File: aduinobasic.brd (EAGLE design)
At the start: 96 parts

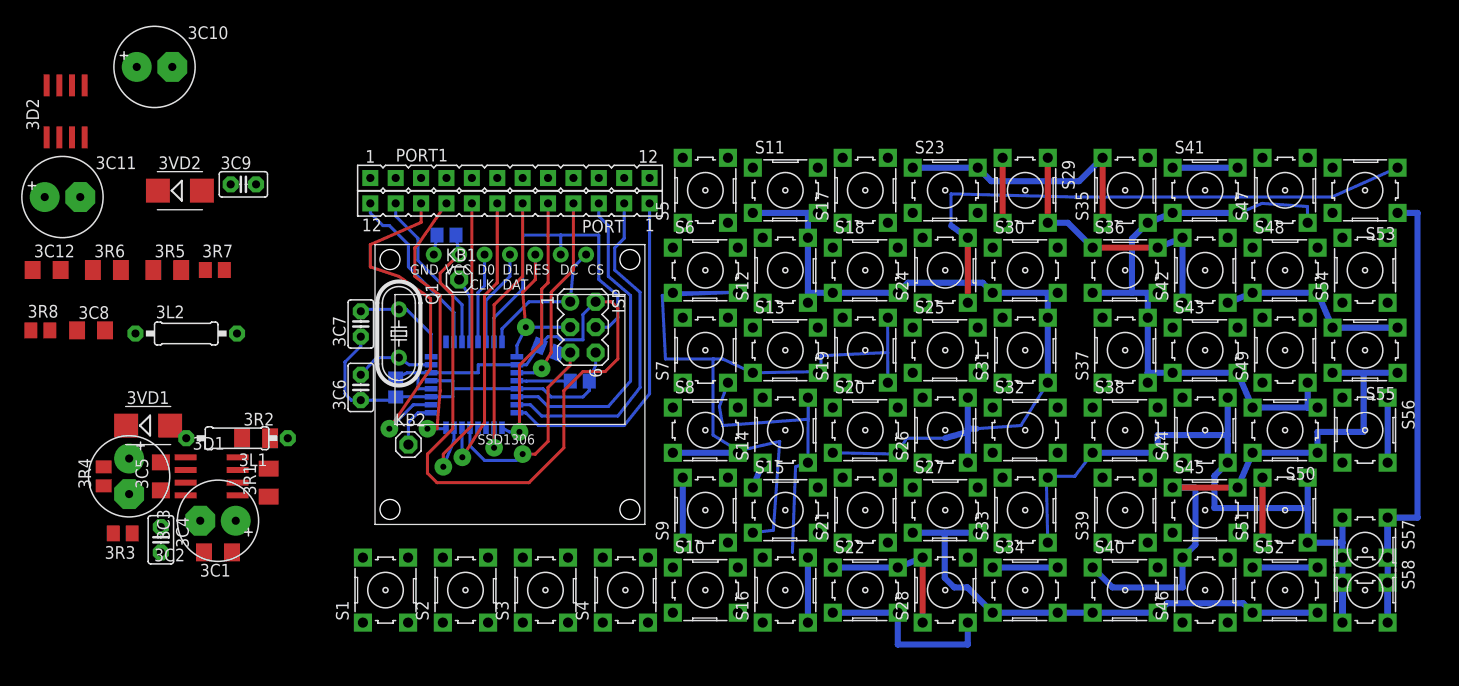
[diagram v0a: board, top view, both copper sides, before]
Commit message: .
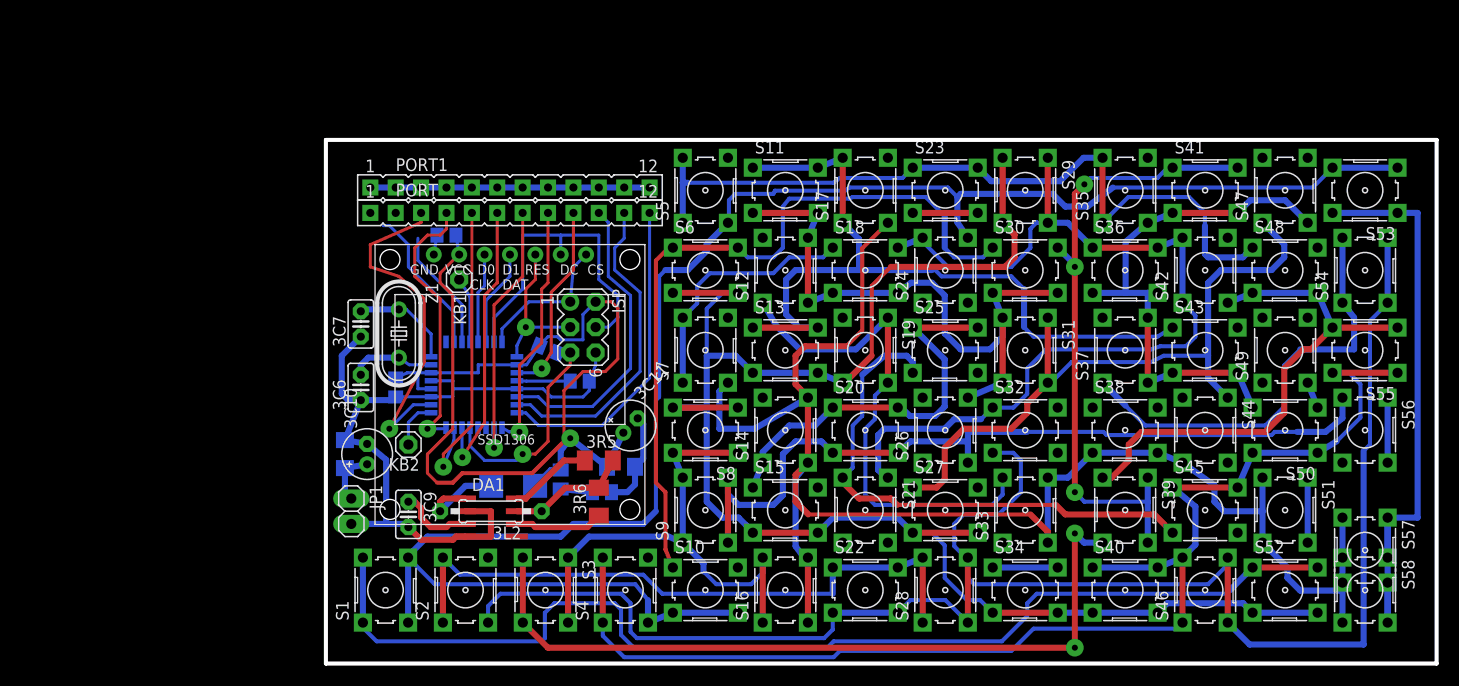
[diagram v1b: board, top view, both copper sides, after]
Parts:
- removed 3C1: 100n, rc-elektronik:C1206
- removed 3C2: 470µ / 10V, HWProgUSB:RCL_E3,5-8
- removed 3C3: 100µ 16V, HWProgUSB:RCL_E3,5-8
- removed 3C4: 1n, rcl:C025-025X050
- removed 3C5: 100n, rcl:C1206
- removed 3D1, 3D2: MC34063AD, mc34063:SOIC8
- removed 3L1: 100uh, rcl:0207/10
- removed 3R1: 0.5-1, rcl:M1206
- removed 3R2: 220, rcl:M1206
- removed 3R3: 2k2, rcl:M0805
- removed 3R4: 20k, rcl:M0805
- removed 3VD1: SS12, diode:SMB
- added DA1: MC34063AD, mc34063:SOIC8
- added JP1: (no value), pinhead:1X02
- 3C10, 3C11: device HWProgUSB:RCL_E3,5-8 -> HWProgUSB:RCL_E2-5
- 3R5: value 220 -> 180
- 3R6: value 0.5-1 -> 1
- 3R7: value 20k -> 3k
- 3R8: value 2k2 -> 1k
- C1, C2, C3: value (none) -> 100n
- Z1: value (none) -> 16Mhz
- moved 3C11 61.3 mm to (56.5, 37.5), turned to 45 degrees
- moved 3C12 60.7 mm to (55.6, 33.3), flipped to the bottom
- moved 3R8 58.5 mm to (53.7, 30.8), flipped to the bottom
- moved 3R6 54.4 mm to (53.3, 29.8), turned to 90 degrees
- moved 3R5 47.2 mm to (53.3, 34.0)
- moved 3VD2 44.5 mm to (44.8, 31.4), flipped to the bottom
- moved 3C10 44.2 mm to (30.2, 34.6), turned to 90 degrees
- moved 3R7 40.5 mm to (49.5, 32.1), flipped to the bottom, turned to 90 degrees
- moved 3C9 36.9 mm to (34.3, 28.6), turned to 270 degrees
- moved 3L2 35.3 mm to (42.5, 28.9), turned to 180 degrees
- moved 3C8 28.3 mm to (27.9, 34.6), flipped to the bottom, turned to 90 degrees
- moved PORT 0.95 mm to (44.5, 58.7), turned to 0 degrees
- moved PORT1 0.95 mm to (44.5, 61.3)
- turned S19 to 270 degrees
- turned S21 to 270 degrees
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- renumbered Q1 to Z1
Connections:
- removed net +12V: 3C11.+, 3C12.2, 3C3.+, 3C5.2, 3R4.2, 3R7.2, 3VD1.C, 3VD2.C
- removed net +5V: 3C1.1, 3C10.+, 3C2.+, 3C8.1, 3D1.6, 3D2.6, 3R1.1, 3R6.1
- removed net N$104: 3D1.8, 3R2.1
- removed net N$105: 3D1.7, 3L1.1, 3R1.2, 3R2.2
- removed net N$106: 3D1.5, 3R3.2, 3R4.1
- removed net N$107: 3D1.1, 3L1.2, 3VD1.A
- removed net N$108: 3C4.1, 3D1.3
- new net V+: 3C10.+, 3C8.1, 3R6.1, DA1.6, JP1.1
- net A0: now also PORT.11; no longer PORT.2
- net A1: now also PORT.12; no longer PORT.1
- net A2: now also PORT.8; no longer PORT.5
- net A3: now also PORT.7; no longer PORT.6
- net A6: now also PORT.9; no longer PORT.4
- net A7: now also PORT.10; no longer PORT.3
- net D0: now also PORT.6; no longer PORT.7
- net D1: now also PORT.5; no longer PORT.8
- net D12: now also S16.2, S3.2, S54.2, S8.2
- net D13: now also S11.2, S13.2, S17.2
- net D14: now also S19.2, S33.2
- net D15: now also S18.2, S21.2, S24.2, S7.2; no longer S24.1
- net D16: now also S20.2, S25.2, S5.2
- net D17: now also S30.2, S39.2, S6.2
- net D18: now also S31.2
- net D19: now also S4.2, S40.2
- net D2: now also PORT.4; no longer PORT.9
- net D23: now also S2.2
- net D26: now also S1.2
- net D3: now also S53.2
- net D4: now also PORT.3; no longer PORT.10
- net D6: now also PORT.1; no longer PORT.12
- net D7: now also PORT.2; no longer PORT.11
- net GND: now also DA1.2, DA1.4, JP1.2, PORT1.1, PORT1.10, PORT1.11, PORT1.12, PORT1.2, PORT1.3, PORT1.4, PORT1.5, PORT1.6, PORT1.7, PORT1.8, PORT1.9; no longer 3C1.2, 3C2.-, 3C3.-, 3C4.2, 3C5.1, 3D1.2, 3D1.4, 3D2.2, 3D2.4, 3R3.1
- net N$5: now also DA1.8; no longer 3D2.8
- net N$6: now also DA1.7; no longer 3D2.7
- net N$7: now also DA1.5; no longer 3D2.5
- net N$8: now also DA1.1; no longer 3D2.1
- net N$9: now also DA1.3; no longer 3D2.3
- net U10: now also S1.4, S10.4, S53.4; no longer S24.3
- net U11: now also S20.4, S9.4
- net U5: now also S3.4, S39.4
- net U6: now also S21.4
- net U7: now also S14.4, S33.4
- net U8: now also S23.4, S46.4, S54.4
- net U9: now also S13.4, S15.4, S19.4, S6.4; no longer S19.3
- net VCC: now also 3C11.+, 3C12.2, 3R7.2, 3VD2.C
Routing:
- net U8: track 18.9 -> 181.0 mm
- net D17: track 6.50 -> 139.6 mm, vias 0 -> 3
- net U10: track 57.0 -> 180.4 mm
- net U5: track 19.5 -> 129.6 mm, vias 0 -> 2
- net D26: track 6.50 -> 113.5 mm
- net D15: track 27.7 -> 118.7 mm
- net D12: track 6.50 -> 97.5 mm
- net D16: track 29.7 -> 118.8 mm
- net D13: track 0.00 -> 79.1 mm
- net GND: track 41.5 -> 115.1 mm
- net D19: track 58.5 -> 128.0 mm
- net D18: track 0.00 -> 69.2 mm
- net U11: track 81.7 -> 144.5 mm
- net U6: track 0.00 -> 53.8 mm
- net D14: track 0.00 -> 51.1 mm
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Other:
- board outline added: 111.1 x 52.4 mm
